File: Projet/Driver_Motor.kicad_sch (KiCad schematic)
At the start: 8 parts, among them J301 Moteur 1, J302 Moteur 1, J303 Conn_01x03, U301 ZXBM5210-S, U302 ZXBM5210-S

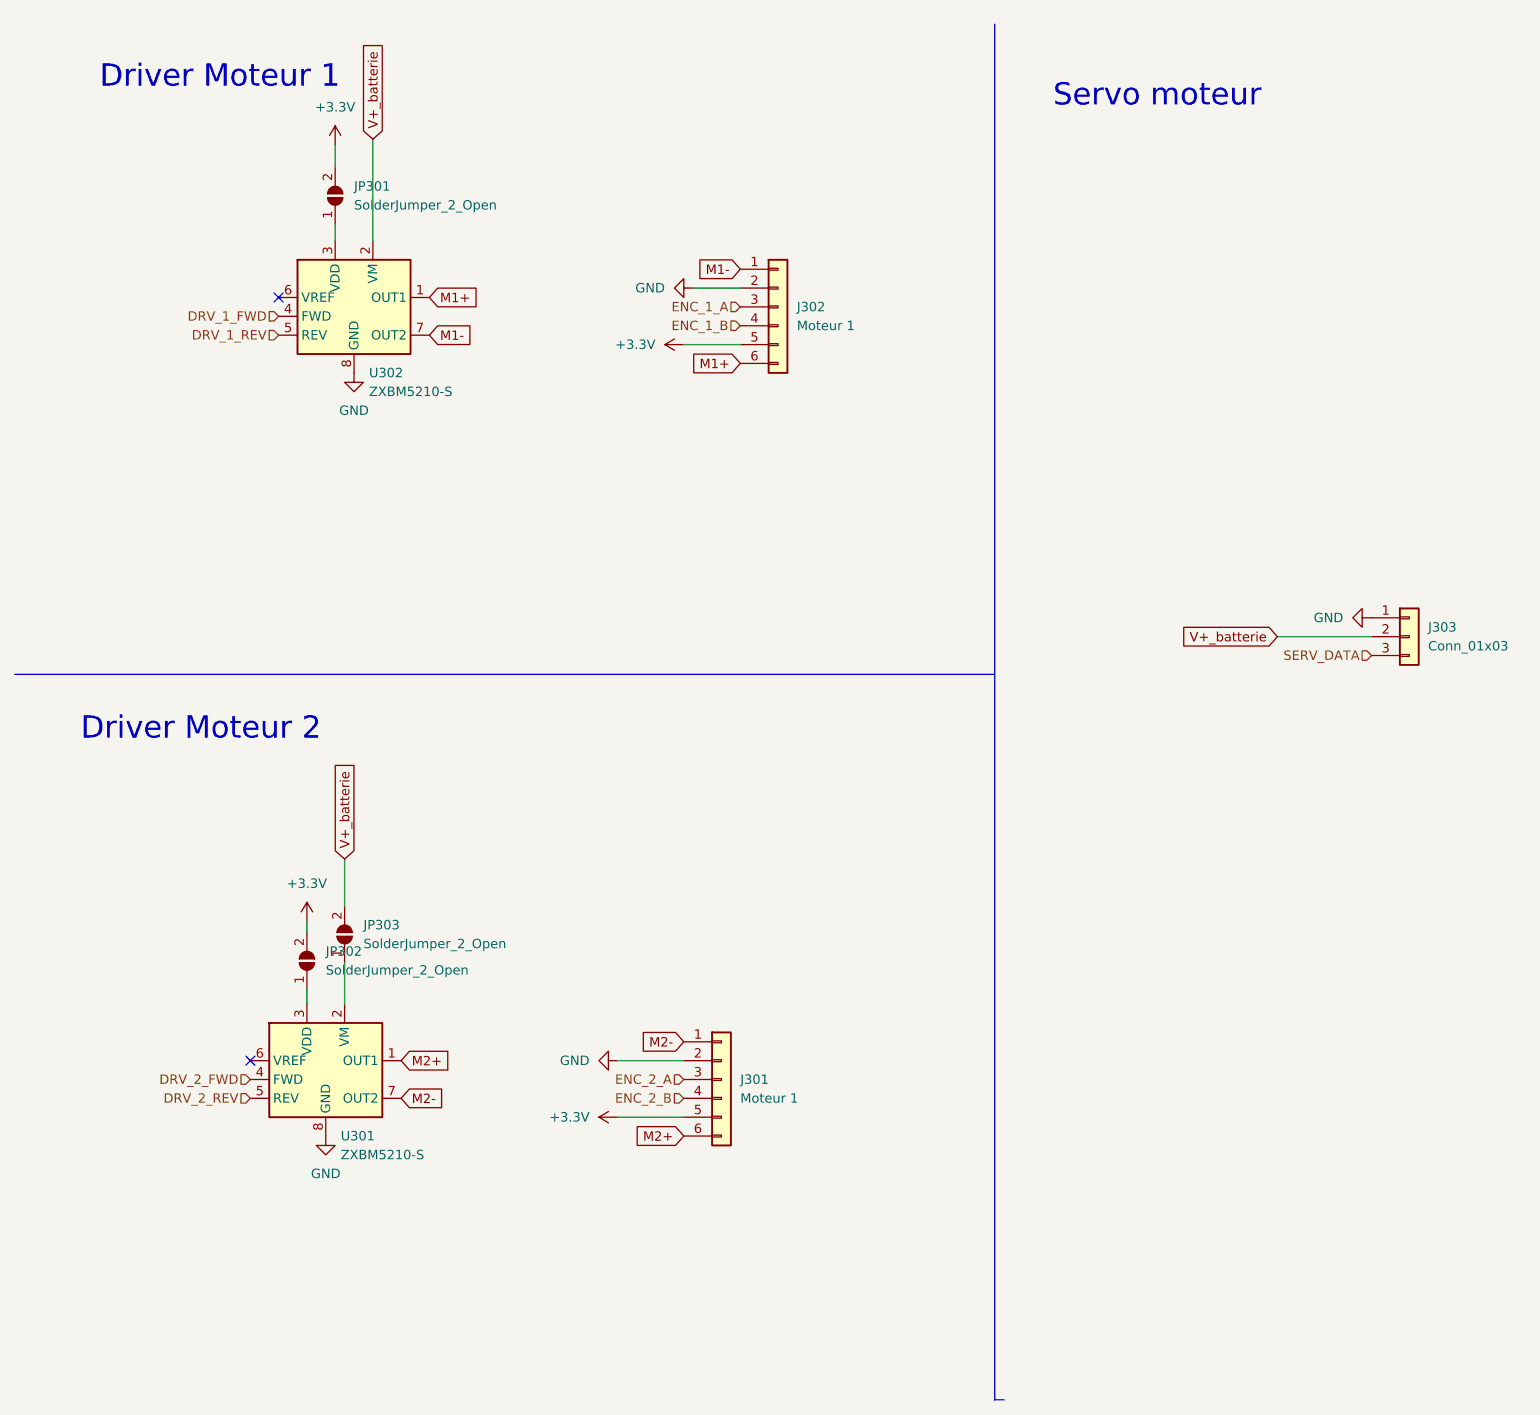
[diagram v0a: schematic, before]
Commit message: placement
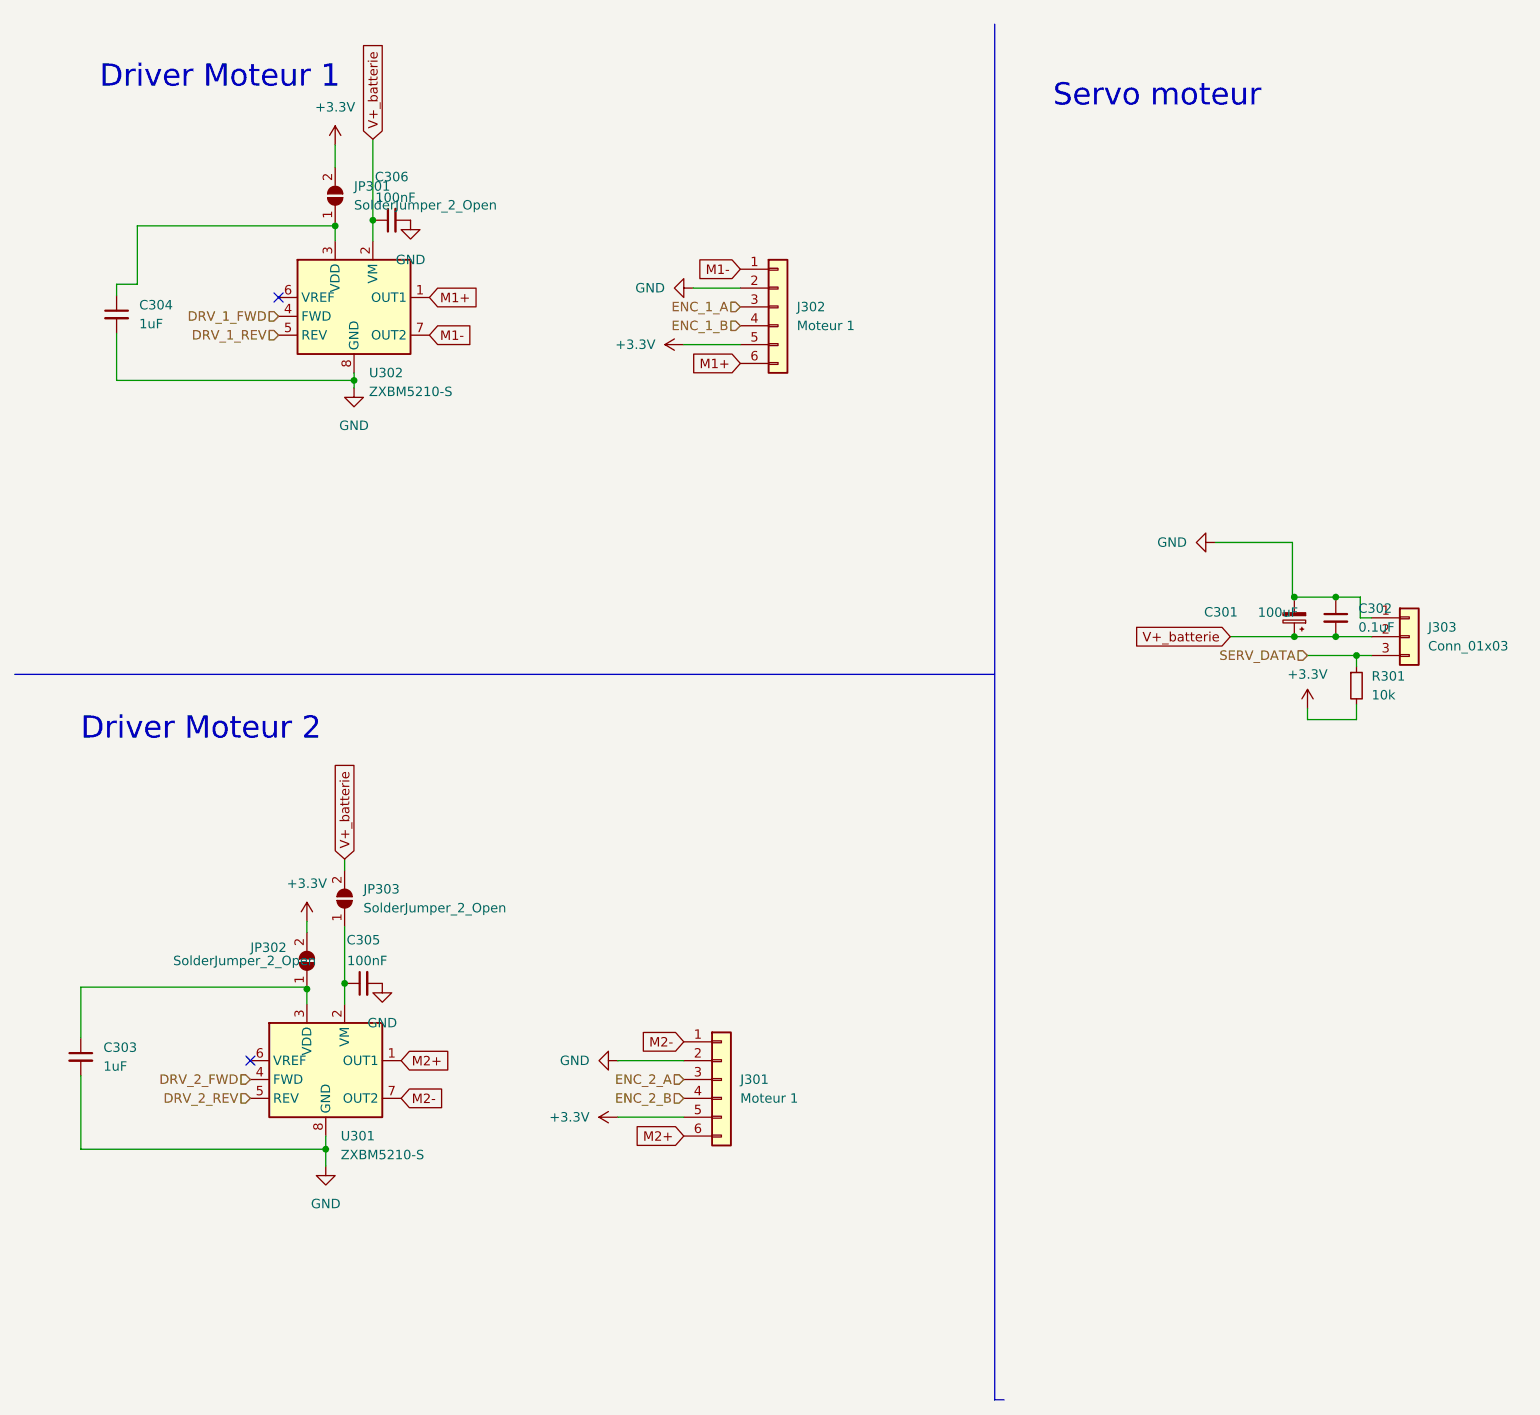
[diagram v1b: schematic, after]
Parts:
- added C301: 100uF, Capacitor_THT:CP_Radial_D6.3mm_P2.50mm, symbol Device:C_Polarized_Small
- added C302: 0.1uF, Capacitor_SMD:C_0603_1608Metric_Pad1.08x0.95mm_HandSolder, symbol Device:C_Small
- added C303, C304: 1uF, Capacitor_SMD:C_0603_1608Metric_Pad1.08x0.95mm_HandSolder, symbol Device:C_Small
- added C305, C306: 100nF, Capacitor_SMD:C_0603_1608Metric_Pad1.08x0.95mm_HandSolder, symbol Device:C_Small
- added R301: 10k, Resistor_SMD:R_0603_1608Metric_Pad0.98x0.95mm_HandSolder, symbol Device:R_Small
- J303: footprint Connector_JST:JST_XH_S3B-XH-A_1x03_P2.50mm_Horizontal -> Connector_JST:JST_XH_B3B-XH-A_1x03_P2.50mm_Vertical
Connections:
- net +3.3V: now also R301.2
- net GND: now also C301.2, C302.1, C303.2, C304.2, C305.2, C306.2
- net SERV_DATA: now also R301.1
- net V+_batterie: now also C301.1, C302.2, C306.1
- net at JP303.1 (A), U301.2 (VM): now also C305.1
- net at JP302.1 (A), U301.3 (VDD): now also C303.1
- net at JP301.1 (A), U302.3 (VDD): now also C304.1
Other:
- moved on the sheet: JP303

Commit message: Routing
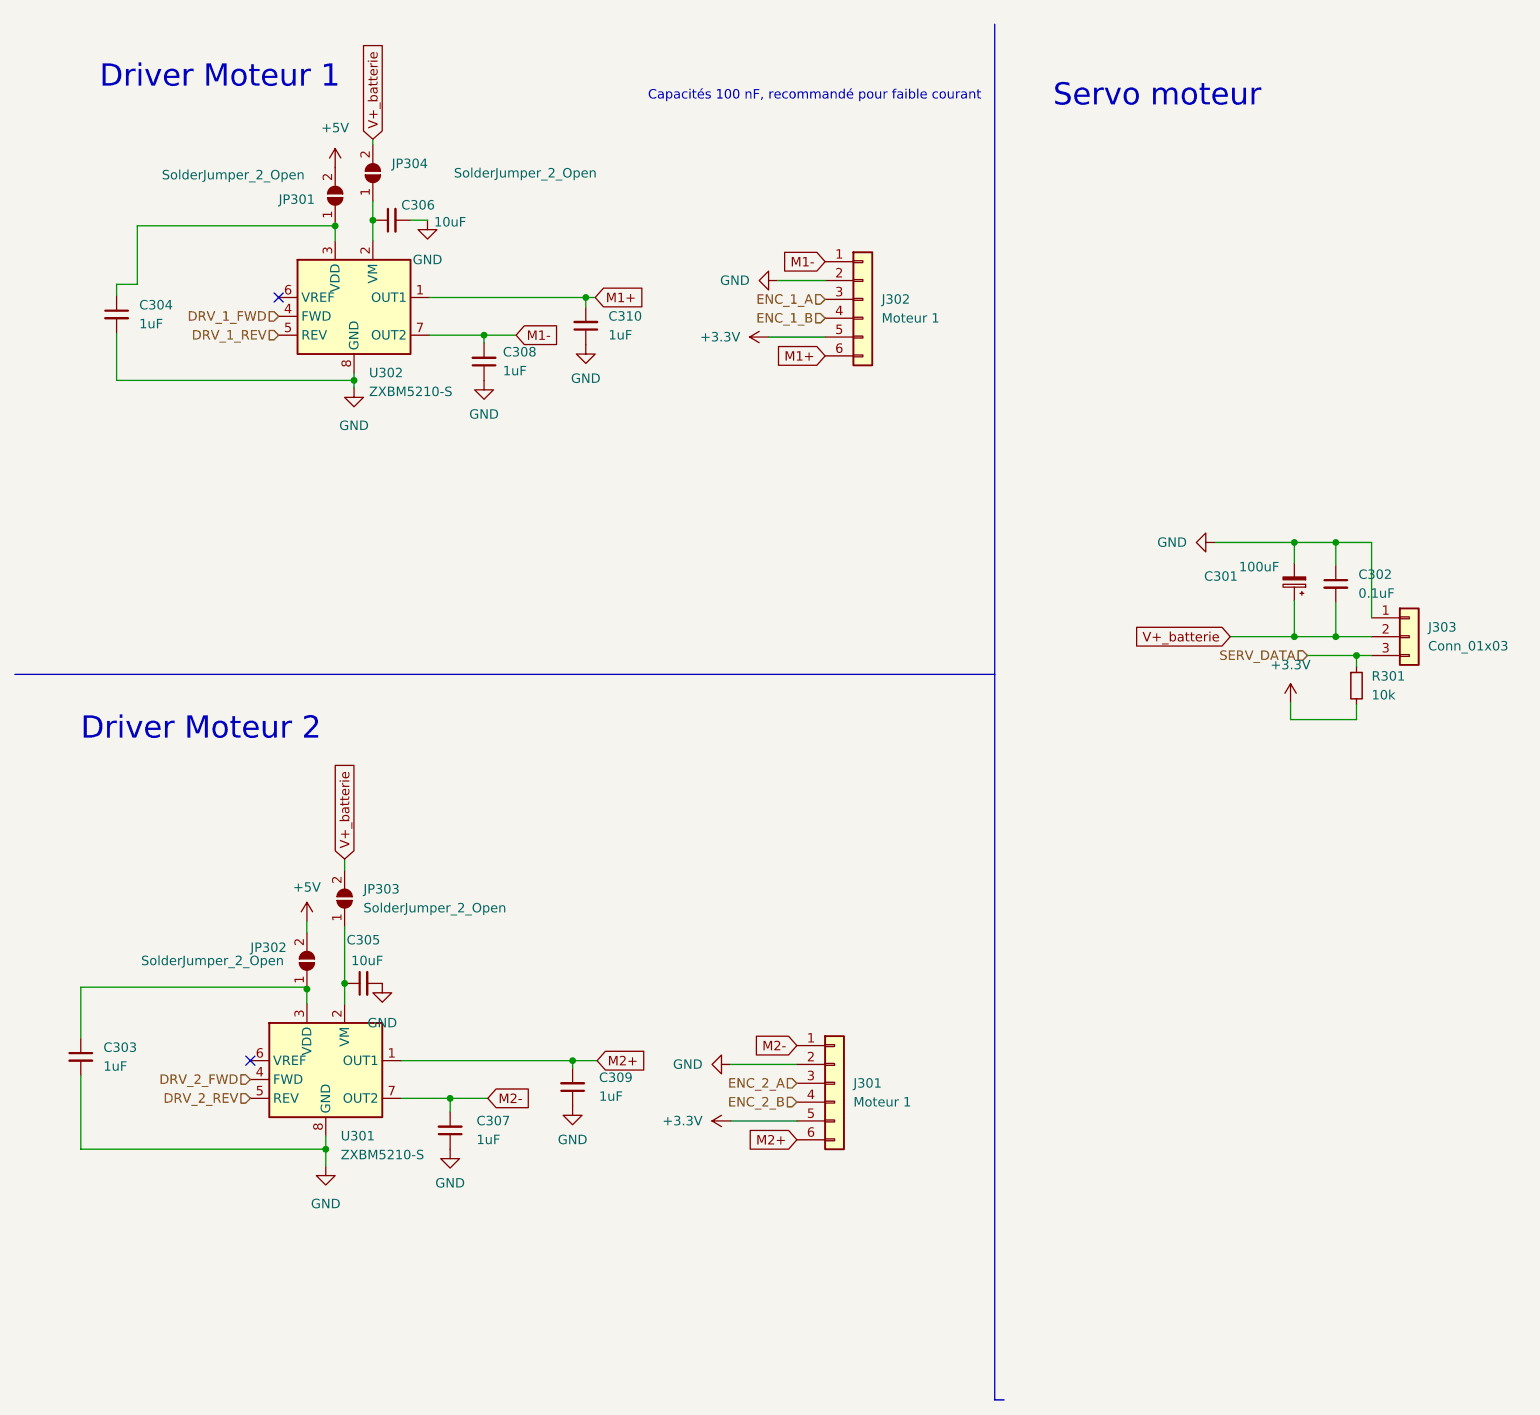
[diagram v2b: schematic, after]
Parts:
- added C307, C308, C309, C310: 1uF, Capacitor_SMD:C_0603_1608Metric_Pad1.08x0.95mm_HandSolder, symbol Device:C_Small
- added JP304: SolderJumper_2_Open, Jumper:SolderJumper-2_P1.3mm_Open_TrianglePad1.0x1.5mm, symbol Jumper:SolderJumper_2_Open
- C305, C306: value 100nF -> 10uF
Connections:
- net +3.3V: no longer JP301.2 (B), JP302.2 (B)
- net GND: now also C307.1, C308.1, C309.1, C310.1
- net M1+: now also C310.2
- net M1-: now also C308.2
- net M2+: now also C309.2
- net M2-: now also C307.2
- net V+_batterie: now also JP304.2 (B); no longer C306.1, U302.2 (VM)
- new net: C306.1, JP304.1 (A), U302.2 (VM)
- new net +5V: JP301.2 (B), JP302.2 (B)
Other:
- note added: "Capacités 100 nF, recommandé pour faible courant"
- moved on the sheet: C301, C302, J301, J302
